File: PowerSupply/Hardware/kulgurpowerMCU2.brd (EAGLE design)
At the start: 102 x 57 mm, 80 parts, among them IC1 TPS77050, IC2 TPS77333DGK, X1 12Mhz, X6 C-GRID-10-70543, X7 C-GRID-10-70543, X8 C-GRID-10-70543, X9 C-GRID-10-70543

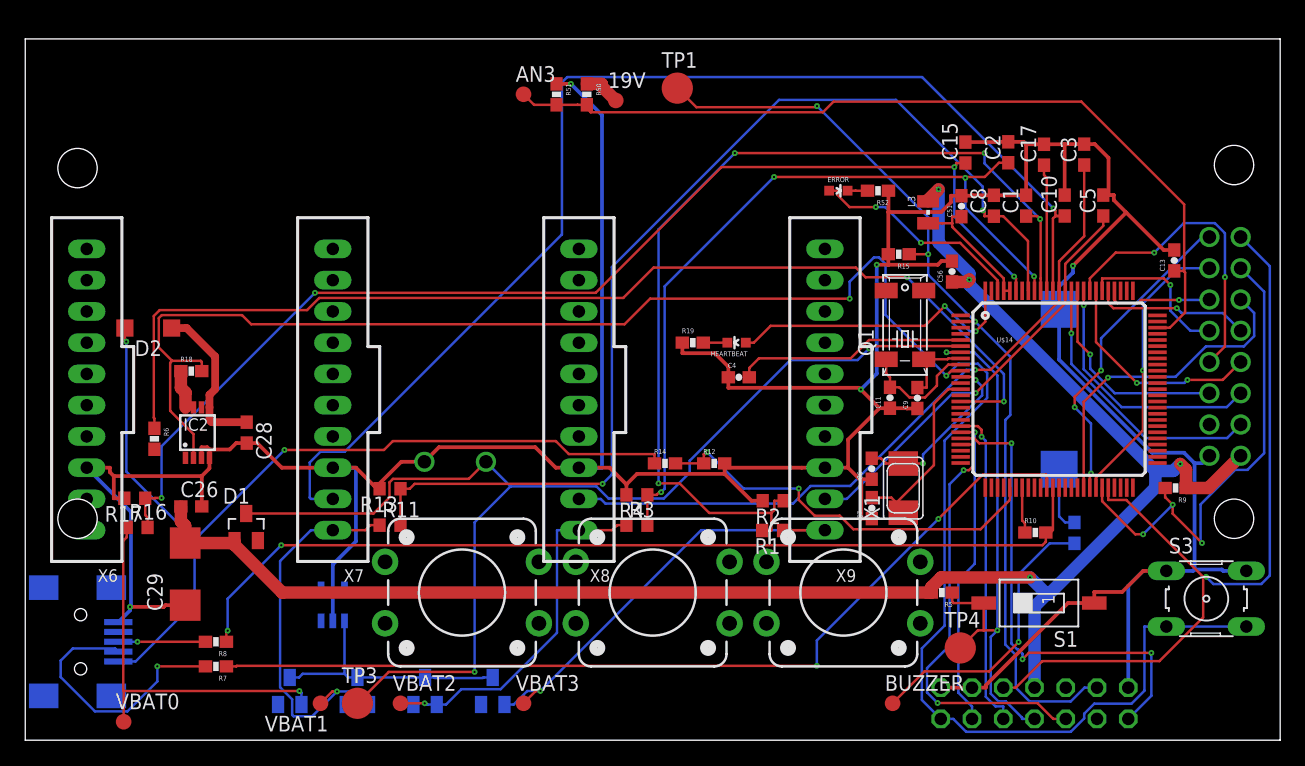
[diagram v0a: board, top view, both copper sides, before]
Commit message: Lot of changes to schematics. A lot.
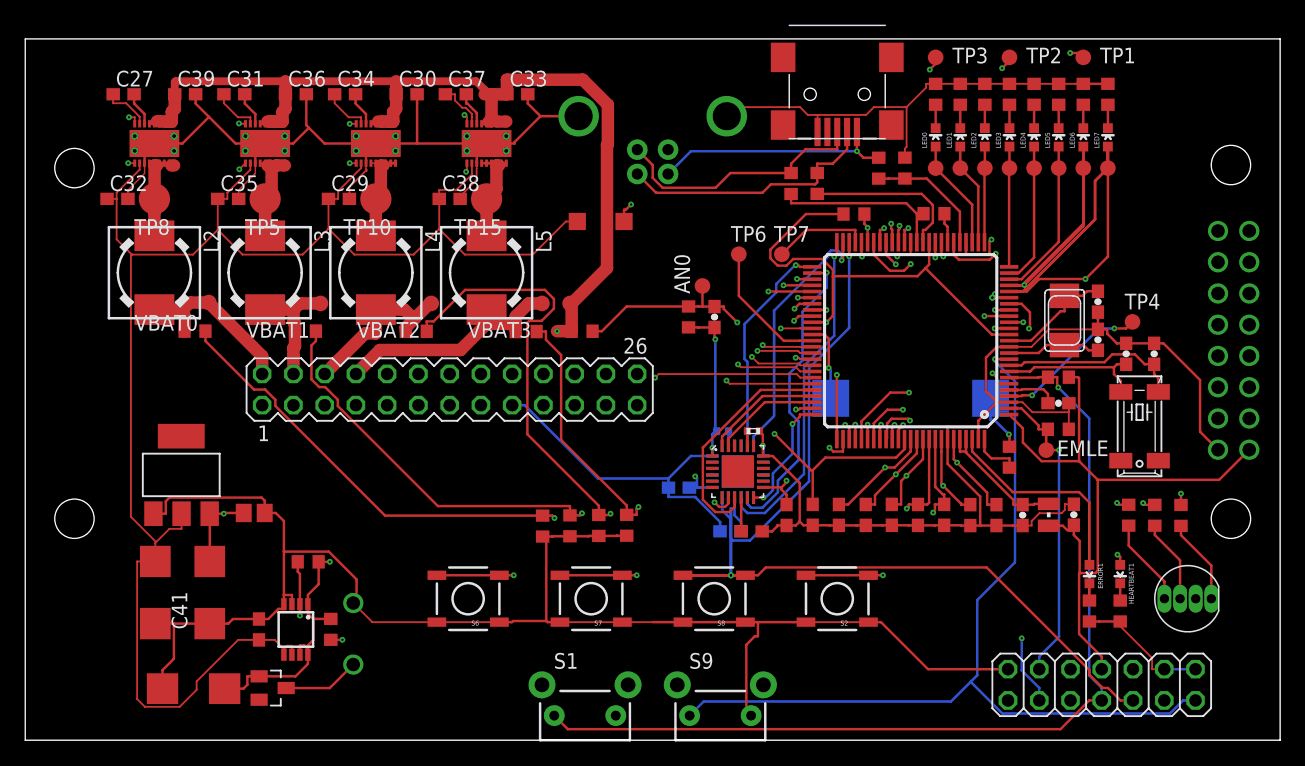
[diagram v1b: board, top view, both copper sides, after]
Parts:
- removed AN3, BUZZER: TPB1,27, testpad:B1,27
- removed C51, C56: 0,1, SparkFun:0603-CAP
- removed CN1: (no value), adafruit:USB-MINIB
- removed D1, D3, D4, D5, D6: BAT54, diode:SOT23
- removed ERROR, HEARTBEAT: (no value), SparkFun:LED-0603
- removed IC1: TPS77050, texas:SOT23-DBV
- removed JP1: (no value), pinhead:2X07
- removed R47, R52: 1k, SparkFun:0603-RES
- removed R50: 100k, SparkFun:0603-RES
- removed R51: 18k, SparkFun:0603-RES
- removed S3: (no value), switch-omron:B3F-10XX
- removed S4, S5: SWITCH-MOMENTARY-212MM, SparkFun-Electromechanical:TACTILE-PTH-12MM
- removed SG2: BUZZERSMD3, SparkFun:BUZZER-CMT1102
- removed X6, X7, X8, X9: C-GRID-10-70543, con-molex:70543-10
- added AN0, EMLE, TP2, TP6, TP7: TPB1,27, testpad:B1,27
- added C12: 0.1, SparkFun:0603-CAP
- added C14: 0,1, SparkFun:0603-CAP
- added C16, C18, C41: (no value), rcl:C/6032-28R
- added C19, C21, C24: 100n, rcl:C0603
- added C20, C25: 2.2nF / 50V, smd-ipc:C0402
- added C23: 1uF/ 26V, resistor:C0805
- added C27, C30, C31, C32, C33, C34, C35, C36, C37, C38, C39: 0.1, rcl:C0603
- added CN2: (no value), adafruit:USB-MINIB
- added D7: BAT54, diode:SOT23
- added D8: LED-RGB-CC-THRUDIFFUSE, SparkFun-LED:LED-RGB-THRU
- added ERROR1, HEARTBEAT1, LED0, LED1, LED2, LED3, LED4, LED5, LED6, LED7: (no value), SparkFun:LED-0603
- added IC3: REG1117-5, burr-brown:SOT223
- added JP2: (no value), pinhead:2X07
- added L1: 4,7uH, wuerth-elektronik:WE-KI_0805_B
- added L2, L4, L5: 4,7uH, inductors:DR73
- added R20, R21, R28, R29, R30, R31, R32, R33, R34: 1k, rcl:R0603
- added R22: 47k, rcl:R0603
- added R23: 100k, rcl:R0603
- added R24, R25: 22r, rcl:R0603
- added R26: 30k, rcl:R0603
- added R27: 17k, rcl:R0603
- added S6: SW1, SparkFun-Electromechanical:TACTILE_SWITCH_SMD
- added S7: SW2, SparkFun-Electromechanical:TACTILE_SWITCH_SMD
- added S8: SW3, SparkFun-Electromechanical:TACTILE_SWITCH_SMD
- added S9: RESET, SparkFun-Electromechanical:TACTILE-PTH-SIDEEZ
- added SG1: BUZZERSMD3, SparkFun:BUZZER-CMT1102
- added SV2: (no value), con-lstb:MA13-2
- added TP10, TP15, TP5, TP8: TPB2,54, testpad:B2,54
- added TPLED0, TPLED1, TPLED2, TPLED3, TPLED4, TPLED5, TPLED6, TPLED7: LED0, testpad:B1,27
- added U$16, U$17, U$18, U$19: CSD97374Q4M, CSD97374Q4M:CSD97374Q4M
- added U$3: ER-OLEDM032-1, oled:ER-OLEDM032-1
- added U1, U2: MPU-6000QFN-24, SparkFun-Sensors:QFN-24-TESTING
- C13: value 0.1 -> 0,1
- C26: value 1uF/6V -> 100n; device resistor:C0603 -> rcl:C0603
- C29: value 47uF/16V -> 0.1; device rcl:C/6032-28R -> rcl:C0603
- L3: device wuerth-elektronik:WE-KI_0805_B -> inductors:DR73
- R10, R15, R19, R5, R6, R9: device SparkFun:0603-RES -> rcl:R0603
- R12: value 30k -> 1k; device SparkFun:0603-RES -> rcl:R0603
- R14: value 17k -> 1k; device SparkFun:0603-RES -> rcl:R0603
- R18: value 47k -> 680k; device SparkFun:0603-RES -> rcl:R0603
- R7, R8: value 22r -> 1k; device SparkFun:0603-RES -> rcl:R0603
- S1: value SWS001 -> PROG; device smd-special:SMS-001 -> SparkFun-Electromechanical:TACTILE-PTH-SIDEEZ
- S2: value SWITCH-MOMENTARY-212MM -> SW4; device SparkFun-Electromechanical:TACTILE-PTH-12MM -> SparkFun-Electromechanical:TACTILE_SWITCH_SMD
- TP1, TP3, TP4: value TPB2,54 -> TPB1,27; device testpad:B2,54 -> testpad:B1,27
- U$1: value ER-OLEDM032-1 -> EDLRD224V3R6C; device oled:ER-OLEDM032-1 -> supercap-EDLRD224V3R6C:EDLRD224V3R6C
- U$2: value EDLRD224V3R6C -> USB+SHIELD; device supercap-EDLRD224V3R6C:EDLRD224V3R6C -> SparkFun-Connectors:USB-B-PTH
- moved R8 75.1 mm to (76.0, 52.5), turned to 270 degrees
- moved R7 74.7 mm to (74.0, 52.5), turned to 270 degrees
- moved TP3 70.5 mm to (74.0, 55.5)
- moved L3 54.1 mm to (19.5, 38.0)
- moved R14 41.0 mm to (80.0, 52.5), turned to 270 degrees
- moved R18 40.7 mm to (53.9, 34.4), turned to 270 degrees
- moved C26 39.7 mm to (53.1, 20.5), flipped to the bottom
- moved S1 38.0 mm to (45.5, 2.00), turned to 0 degrees
- moved D2 37.8 mm to (46.8, 42.2), turned to 0 degrees
- moved R12 37.2 mm to (78.0, 52.5), turned to 270 degrees
- moved C3 35.4 mm to (66.1, 18.3), turned to 270 degrees
- moved VBAT0 34.8 mm to (14.9, 35.6), turned to 180 degrees
- moved C5 34.5 mm to (64.0, 18.3), turned to 270 degrees
- moved R9 34.3 mm to (67.4, 42.8), turned to 0 degrees
- moved R17 33.2 mm to (42.1, 17.4), turned to 270 degrees
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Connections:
- removed net !SS1: JP1.9, U$14.19
- removed net !SS12: U$14.75
- removed net !SS3: JP1.5, U$14.22
- removed net !SS5: U$14.64
- removed net !SS9: U$14.56
- removed net +5V: C28.1, D2.C, IC2.5, IC2.6
- removed net 19V: 19V.TP, R50.1
- removed net AN3: AN3.TP, C13.1, R50.2, R51.2, U$14.73
- removed net EN_PANDA: R47.1, SG2.1
- removed net N$32: U$14.71
- removed net N$33: U$14.70
- removed net N$34: U$14.65
- removed net N$35: U$14.63
- removed net N$43: JP1.6
- removed net SCK0: U$14.26
- removed net SCK1: JP1.1, U$14.21
- removed net SCK12: U$14.78
- removed net SCK3: U$14.24
- removed net SCK5: U$14.69
- removed net SCK6: U$14.16
- removed net SCK9: U$14.55
- removed net SCL0: U$14.34
- removed net SCL5: U$14.67
- removed net SDA0: U$14.33
- removed net SMISO0: U$14.27
- removed net SMISO1: JP1.11, U$14.20
- removed net SMISO12: U$14.76
- removed net SMISO3: U$14.23
- removed net SMISO5: U$14.68
- removed net SMISO6: U$14.17
- removed net SMISO9: U$14.54
- removed net SMOSI0: U$14.28
- removed net SMOSI12: U$14.77
- removed net SMOSI3: U$14.25
- removed net SMOSI5: U$14.66
- removed net SMOSI6: U$14.18
- removed net SMOSI9: U$14.53
- removed net VBATT: D1.3, TP3.TP, U$14.6, U$2.P
- new net !SKIP0: U$14.69, U$16.P$1
- new net !SKIP1: U$14.68, U$17.P$1
- new net !SKIP2: U$14.67, U$18.P$1
- new net !SKIP3: U$14.65, U$19.P$1
- new net !SW1: S6.3, S6.4, U$14.17
- new net !SW2: S7.3, S7.4, U$14.18
- new net !SW3!/TMS: JP2.9, S8.3, S8.4, U$14.19
- new net !SW4!/TDI: S2.3, S2.4, U$14.20
- new net !TRST: JP2.3, U$14.16
- new net +19V: 19V.TP, C30.1, C33.1, C36.1, C39.1, R23.2, SV2.14, SV2.16, U$16.P$5A, U$16.P$5B, U$16.P$5C, U$16.P$5D, U$16.P$5E, U$16.P$5F, U$17.P$5A, U$17.P$5B, U$17.P$5C, U$17.P$5D, U$17.P$5E, U$17.P$5F, U$18.P$5A, U$18.P$5B, U$18.P$5C, U$18.P$5D, U$18.P$5E, U$18.P$5F, U$19.P$5A, U$19.P$5B, U$19.P$5C, U$19.P$5D, U$19.P$5E, U$19.P$5F
- new net 5V: C16.+, C28.1, C29.1, C32.1, C35.1, C38.1, D2.C, IC2.5, IC2.6, IC3.2, U$16.P$2, U$17.P$2, U$18.P$2, U$19.P$2
- new net AN0: AN0.TP, C12.1, R18.1, R23.1, U$14.76
- new net BAT0_EN: SV2.9, U$14.59
- new net BAT1_EN: SV2.11, U$14.58
- new net BAT2_EN: SV2.13, U$14.57
- new net BAT3_EN: SV2.15, U$14.56
- new net CPOUT1: C20.1, U1.20
- new net CPOUT2: C25.1, U2.20
- new net CS: U$14.74, U1.8
- new net CS5: U$14.52, U2.8
- new net EN_PANDA1: R19.1, SG1.1
- new net INT_GYRO1: U$14.75, U1.12
- new net INT_GYRO2: U$14.48, U2.12
- new net LED0: LED0.A, TPLED0.TP, U$14.28
- new net LED1: LED1.A, TPLED1.TP, U$14.27
- new net LED2: LED2.A, TPLED2.TP, U$14.26
- new net LED3: LED3.A, TPLED3.TP, U$14.25
- new net LED4: LED4.A, TPLED4.TP, U$14.24
- new net LED5: LED5.A, TPLED5.TP, U$14.23
- new net LED6/TDO: JP2.5, LED6.A, TPLED6.TP, U$14.22
- new net LED7/TCK: JP2.1, JP2.11, LED7.A, TPLED7.TP, U$14.21
- new net LED_BLUE: R34.2, U$14.33
- new net LED_GREEN: R33.2, U$14.31
- new net LED_RED: R32.2, U$14.29
- new net MISO: U$14.71, U1.9
- new net MISO5: U$14.50, U2.9
- new net MOSI: U$14.72, U1.24
- new net MOSI5: U$14.49, U2.24
- new net N$10: LED3.C, R14.2
- new net N$11: LED4.C, R28.2
- new net N$12: LED5.C, R29.2
- new net N$13: LED6.C, R30.2
- new net N$14: LED7.C, R31.2
- new net N$15: D8.3, R33.1
- new net N$18: C37.1, U$19.P$7
- new net N$20: C37.2, U$19.P$6
- new net N$22: C27.1, U$16.P$7
- new net N$23: C27.2, U$16.P$6
- new net N$24: C34.1, U$18.P$7
- new net N$25: C34.2, U$18.P$6
- new net N$26: TP1.TP, U$14.39
- new net N$28: TP3.TP, U$14.41
- new net N$30: TP6.TP, U$14.63
- new net N$7: ERROR1.C, R21.2
- new net OUT1_EN: SV2.18, U$14.55
- new net OUT2_EN: SV2.20, U$14.54
- new net OUT3_EN: SV2.22, U$14.53
- new net OUT4_EN: SV2.24, U$14.78
- new net OUT5_EN: SV2.26, U$14.77
- new net PWM0: U$14.70, U$16.P$8
- new net PWM1: U$14.66, U$17.P$8
- new net PWM2: U$14.64, U$18.P$8
- new net PWM3: U$14.61, U$19.P$8
- new net REGOUT1: C19.1, U1.10
- new net REGOUT2: C24.1, U2.10
- new net SCLK: U$14.73, U1.23
- new net SCLK5: U$14.51, U2.23
- new net SUPERCAP: D7.3, U$1.P, U$14.6
- new net USB0_VBUS: R26.1, R27.2, U$14.30
- new net V+: C23.1, C41.+, IC3.3, SV2.12
- new net VSW0: L2.1, TP8.TP, U$16.P$4A, U$16.P$4B, U$16.P$4C, U$16.P$4D, U$16.P$4E, U$16.P$4F
- new net VSW1: L3.1, TP5.TP, U$17.P$4A, U$17.P$4B, U$17.P$4C, U$17.P$4D, U$17.P$4E, U$17.P$4F
- new net VSW2: L4.1, TP10.TP, U$18.P$4A, U$18.P$4B, U$18.P$4C, U$18.P$4D, U$18.P$4E, U$18.P$4F
- new net VSW3: L5.1, TP15.TP, U$19.P$4A, U$19.P$4B, U$19.P$4C, U$19.P$4D, U$19.P$4E, U$19.P$4F
- net !OLED_CS: now also JP2.10, U$3.P$16; no longer JP1.10, U$1.P$16
- net !OLED_DC: now also U$3.P$14; no longer U$1.P$14
- net !OLED_RD: now also U$3.P$12; no longer U$1.P$12
- net !OLED_RESET: now also U$3.P$15; no longer U$1.P$15
- net !OLED_WR: now also U$3.P$13; no longer U$1.P$13
- net !RESET: now also JP2.13, R22.2, S9.1; no longer JP1.13, R18.2, S3.3, S3.4
- net +3V3: now also C14.1, C18.+, C21.1, D7.1, JP2.8, L1.1, R22.1, U$3.P$2, U1.13, U2.13; no longer C29.+, C56.1, D1.1, JP1.8, L3.1, R18.1, U$1.P$2
- net AVCC0: now also C13.1, L1.2; no longer C51.1, L3.2
- net BUZZER: now also R19.2, U$14.100; no longer BUZZER.TP, R47.2
- net D+: now also CN2.D+, R25.2, U$2.D+; no longer CN1.D+, R8.2
- net D-: now also CN2.D-, R24.2, U$2.D-; no longer CN1.D-, R7.2
- net D0: now also U$3.P$4; no longer U$1.P$4
- net D1: now also U$3.P$5; no longer U$1.P$5
- net D2: now also U$3.P$6; no longer U$1.P$6
- net D3: now also U$3.P$7; no longer U$1.P$7
- net D4: now also U$3.P$8; no longer U$1.P$8
- net D5: now also U$3.P$9; no longer U$1.P$9
- net D6: now also U$3.P$10; no longer U$1.P$10
- net D7: now also U$3.P$11; no longer U$1.P$11
- net EMLE: now also EMLE.TP, JP2.4; no longer JP1.4, TP1.TP
- net ERROR: now also ERROR1.A; no longer ERROR.A
- net GND: now also C12.2, C14.2, C16.-, C18.-, C19.2, C20.2, C21.2, C23.2, C24.2, C25.2, C29.2, C30.2, C32.2, C33.2, C35.2, C36.2, C38.2, C39.2, C41.-, CN2.GND, D8.2, IC3.1, JP2.12, JP2.14, JP2.2, R12.1, R14.1, R18.2, R20.1, R21.1, R26.2, R28.1, R29.1, R30.1, R31.1, R7.1, R8.1, S1.2, S2.1, S2.2, S6.1, S6.2, S7.1, S7.2, S8.1, S8.2, S9.2, SG1.2, SV2.10, SV2.17, U$1.N, U$16.P$3, U$16.PAD@1, U$17.P$3, U$17.PAD@1, U$18.P$3, U$18.PAD@1, U$19.P$3, U$19.PAD@1, U$2.GND, U$2.S1, U$2.S2, U$3.P$1, U1.1, U1.18, U2.1, U2.18; no longer C29.-, C51.2, C56.2, CN1.GND, IC1.2, JP1.12, JP1.14, JP1.2, R12.2, R19.1, R51.1, R52.1, S1.1, S3.1, S3.2, SG2.2, U$1.P$1, U$2.N, X6.3, X7.3, X8.3, X9.3
- net HEARTBEAT: now also HEARTBEAT1.A, U$14.34; no longer HEARTBEAT.A, U$14.100
- net IBAT0_AD: now also SV2.19; no longer X6.2
- net IBAT1_AD: now also SV2.21; no longer X7.2
- net IBAT2_AD: now also SV2.23; no longer X8.2
- net IBAT3_AD: now also SV2.25; no longer X9.2
- net MD: now also JP2.7, S1.1; no longer JP1.7, S1.2, TP4.TP
- net N$17: now also D8.4, R34.1; no longer HEARTBEAT.C, R19.2
- net N$19: now also C31.1, U$17.P$7; no longer U$14.31
- net N$2: now also LED0.C, R7.2; no longer R12.1, R14.2, U$14.30
- net N$21: now also C31.2, U$17.P$6; no longer U$14.4
- net N$27: now also TP2.TP, U$14.40; no longer U$14.74
- net N$29: now also TP4.TP, U$14.4; no longer ERROR.C, R52.2
- net N$31: now also TP7.TP, U$14.47; no longer U$14.72
- net N$4: now also D8.1, R32.1; no longer D3.3, D4.3, D5.3, D6.3, IC1.1
- net N$5: now also HEARTBEAT1.C, R20.2; no longer IC1.3
- net N$8: now also LED1.C, R8.2; no longer IC1.5
- net N$9: now also LED2.C, R12.2; no longer IC1.4
- net USB0_DM: now also R24.1; no longer R7.1
- net USB0_DP: now also R25.1; no longer R8.1
- net VBAT0: now also L2.2, SV2.1, SV2.2; no longer D3.1, X6.1
- net VBAT1: now also L3.2, SV2.3, SV2.4; no longer D4.1, X7.1
- net VBAT2: now also L4.2, SV2.5, SV2.6; no longer D5.1, X8.1
- net VBAT3: now also L5.2, SV2.7, SV2.8; no longer D6.1, X9.1
- net VBUS: now also CN2.VBUS, R27.1, U$2.VBUS; no longer CN1.VBUS, R14.1
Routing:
- net GND: track 332.5 -> 498.2 mm
- net 5V: track 0.00 -> 132.4 mm
- net VBATT: track 94.3 -> 0.00 mm, vias 2 -> 0
- net +19V: track 0.00 -> 92.6 mm, vias 0 -> 1
- net !SW3!/TMS: track 0.00 -> 78.8 mm, vias 0 -> 1
- net AN3: track 70.8 -> 0.00 mm
- net SUPERCAP: track 0.00 -> 70.0 mm, vias 0 -> 1
- net LED7/TCK: track 0.00 -> 68.6 mm, vias 0 -> 1
- net +3V3: track 144.3 -> 210.6 mm
- net PWM0: track 0.00 -> 65.5 mm, vias 0 -> 2
- net !SKIP0: track 0.00 -> 63.7 mm, vias 0 -> 2
- net USB0_DP: track 77.0 -> 14.2 mm, vias 2 -> 0
- net IBAT1_AD: track 98.2 -> 35.9 mm
- net USB0_DM: track 75.4 -> 13.2 mm, vias 2 -> 0
- net PWM1: track 0.00 -> 59.8 mm, vias 0 -> 2
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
